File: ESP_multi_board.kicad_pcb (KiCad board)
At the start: 2 copper layers, 24 parts, among them P101 CONN_01X02, P102 CONN_01X06, P103 CONN_01X02, P104 CONN_01X06, P105 CONN_01X12, P106 CONN_01X03, P107 CONN_I2C_MPU6050, P108 CONN_PINES_DIG, SW101 SW_PUSH_SMALL, SW102 SWITCH_INV, U1 LD1117S33TR, U101 L293DD, U102 ESP-12, U103 MAX11605EEE+, U104 MCP23008

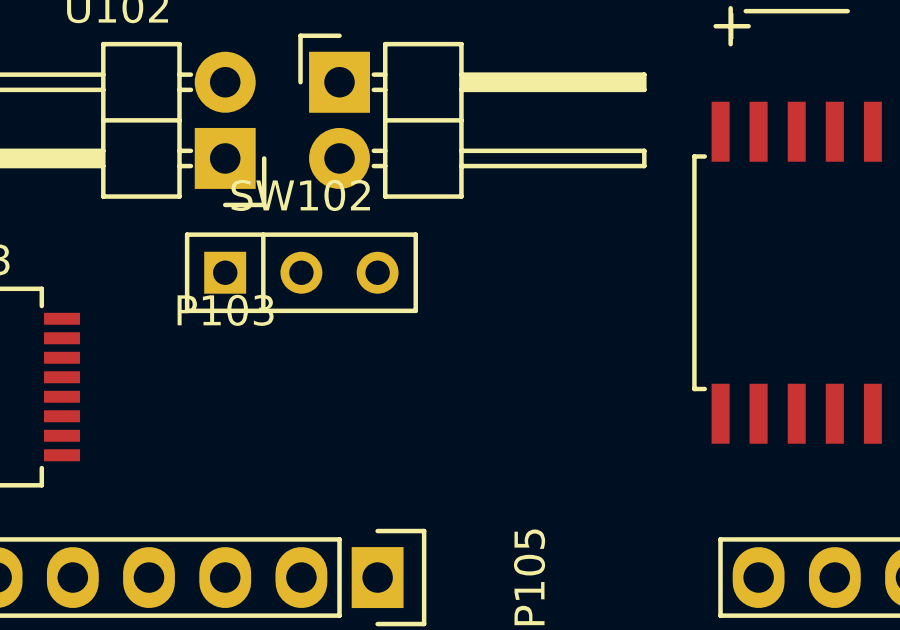
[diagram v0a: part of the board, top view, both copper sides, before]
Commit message: routing
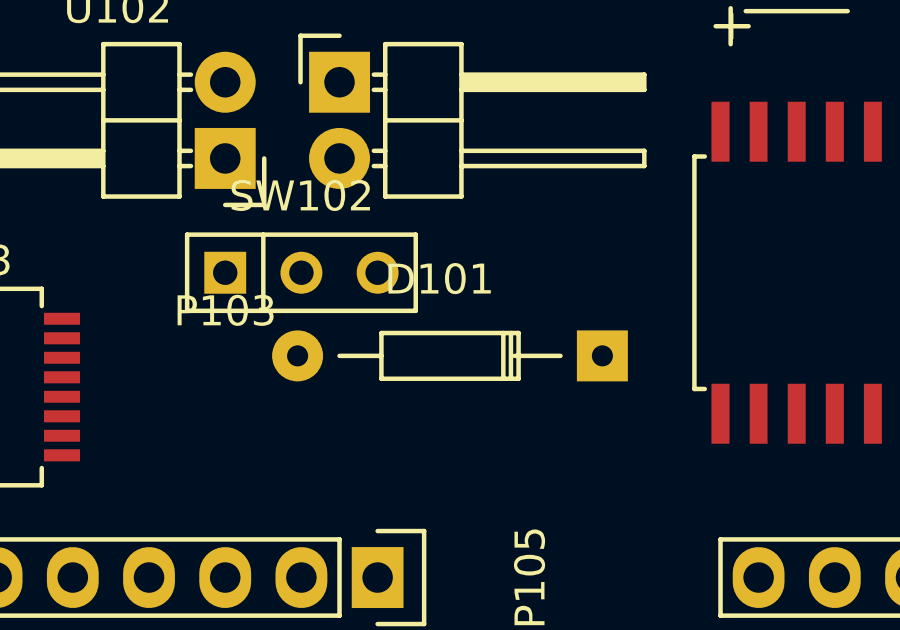
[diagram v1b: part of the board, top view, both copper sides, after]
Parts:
- added D101: D, Diodes_ThroughHole:Diode_DO-35_SOD27_Horizontal_RM10, F.Cu at (162.4, 86.6)
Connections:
- P101 pad 2: Net-(P101-Pad2) -> Net-(D101-Pad1)
- SW102 pad 2: Net-(P101-Pad2) -> Net-(D101-Pad2)
